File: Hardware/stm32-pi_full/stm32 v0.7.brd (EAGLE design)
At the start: 131.4 x 105.8 mm, 221 parts, among them J1 SOLDERJUMPERNO, Q1 MMBT3906, Q2 MMBT3904, Q3 MMBT3904, U1 ESP32-WROOM-32D

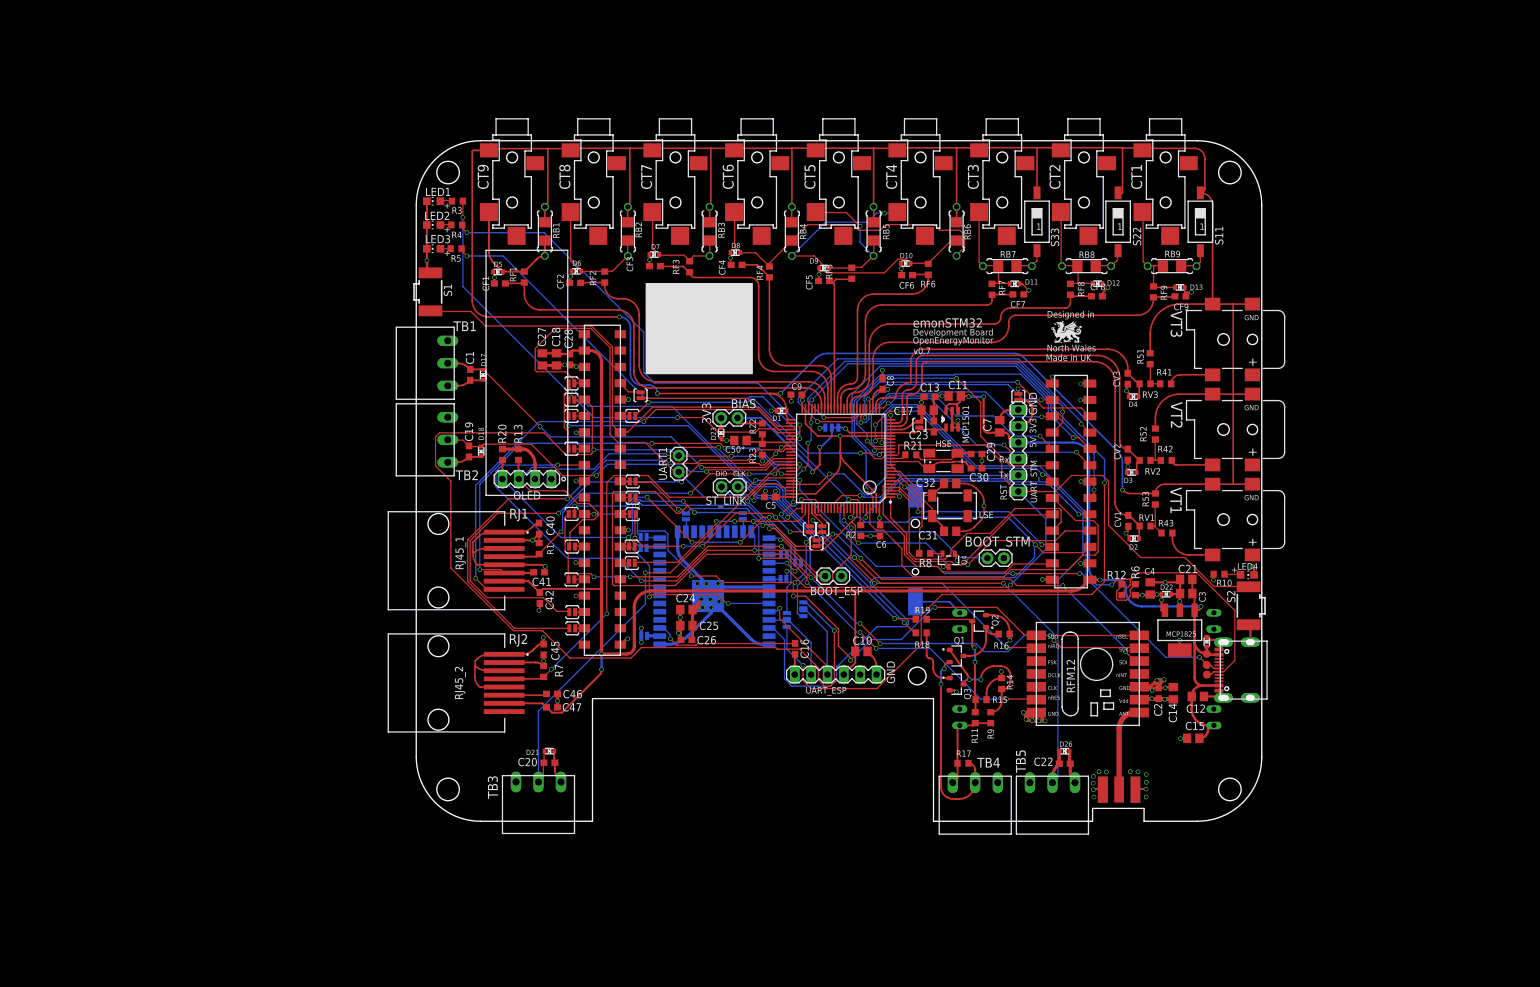
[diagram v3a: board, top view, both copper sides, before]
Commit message: update dec2019
v0.7 gerbers sent to manf.
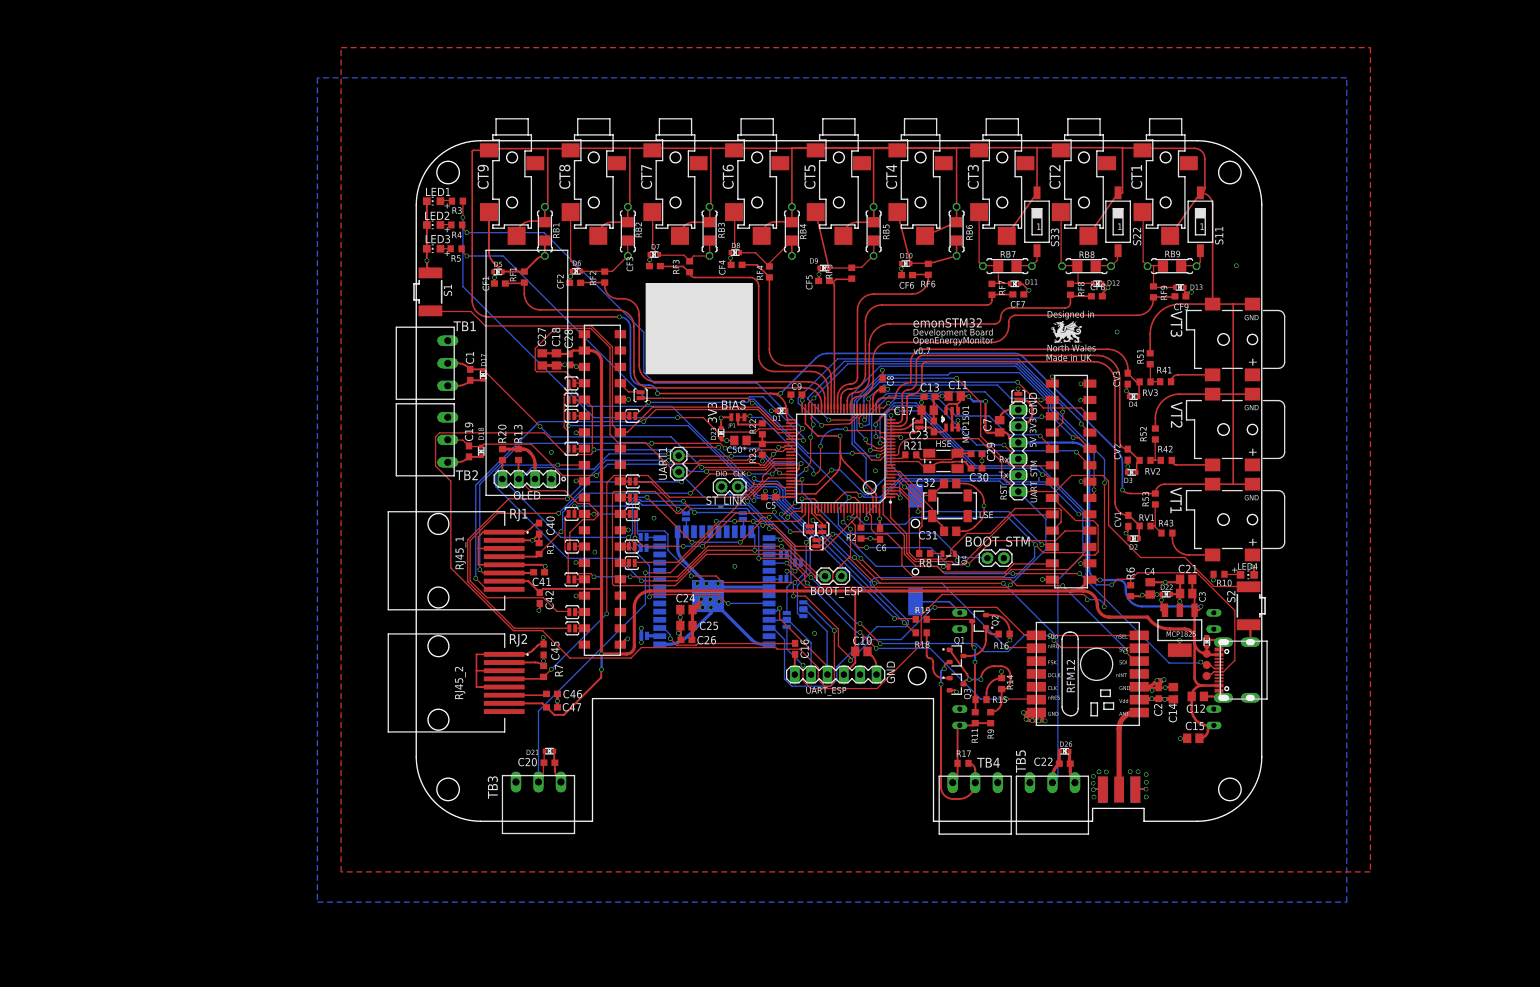
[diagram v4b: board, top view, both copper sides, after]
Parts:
- removed BIAS_IN: (no value), SparkFun:1X02
- removed R12: 330R, rcl:R0603
- R6: value 1k -> 1.5k
- moved RB13 25.6 mm to (84.0, 91.7)
- moved RB15 25.6 mm to (58.4, 91.7)
- moved JP1 14.7 mm to (50.0, 62.8), flipped to the top, turned to 0 degrees
- moved R6 0.76 mm to (111.1, 35.8)
- moved C6 0.53 mm to (72.1, 44.7)
- moved R2 0.40 mm to (69.1, 44.8)
- moved R41 0.33 mm to (116.5, 68.3)
- moved RV3 0.30 mm to (113.3, 68.3)
- moved TP5 0.21 mm to (122.9, 22.6)
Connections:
- removed net N$7: R12.1, R6.2
- net +3V3: no longer BIAS_IN.1
- net BIAS: now also CT1.P$4, CT2.P$4, CT3.P$4, CT4.P$4, CT5.P$4, CT6.P$4, CT7.P$4, CT8.P$4, CT9.P$4
- net D+: now also R6.2; no longer R12.2
- net N$12: no longer BIAS_IN.2
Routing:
- net BIAS: track 467.4 -> 567.2 mm
- net N$40: track 49.2 -> 18.0 mm, vias 1 -> 0
- net N$38: track 50.9 -> 20.2 mm
- net N$12: track 28.4 -> 4.99 mm, vias 2 -> 0
- net VREF+: track 18.3 -> 41.5 mm, vias 1 -> 4
- net +5V: track 302.1 -> 324.4 mm
- net N$7: track 7.29 -> 0.00 mm
- net N$39: track 23.4 -> 19.1 mm, vias 1 -> 0
- net USART3_RX: track 141.6 -> 145.4 mm, vias 3 -> 5
- net +3V3: track 85.1 -> 88.6 mm
- net GND: track 367.0 -> 365.0 mm, vias 80 -> 89
- net DS18B20_2_RJ45: track 80.4 -> 82.3 mm
- net CT3_EX: track 36.2 -> 38.0 mm
- net BOOT0: track 73.8 -> 75.1 mm
- net D+: track 118.7 -> 117.4 mm
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- added copper zone on layer 1, net GND
- added copper zone on layer 16, net GND
